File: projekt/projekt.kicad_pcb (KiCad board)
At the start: 2 copper layers, 28 parts, among them J1 Conn_01x05, J2 Conn_01x04, J4 87583-0010RHLF, J5 10118192-0001LF, U1 MAX17048G_T10, U2 TPS61022RWUT, U3 MCP73871-2CCI_ML

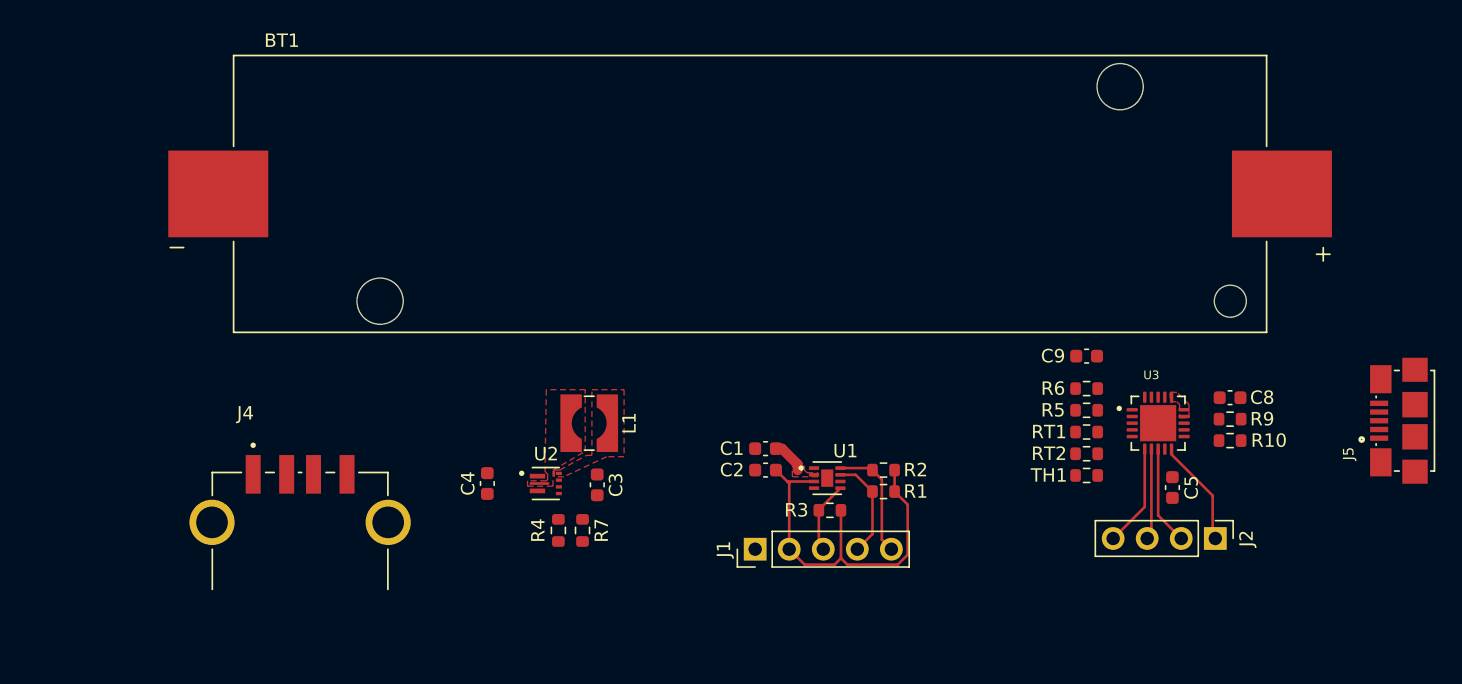
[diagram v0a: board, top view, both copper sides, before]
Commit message: MAIN: wersja pierwsza 19.04.
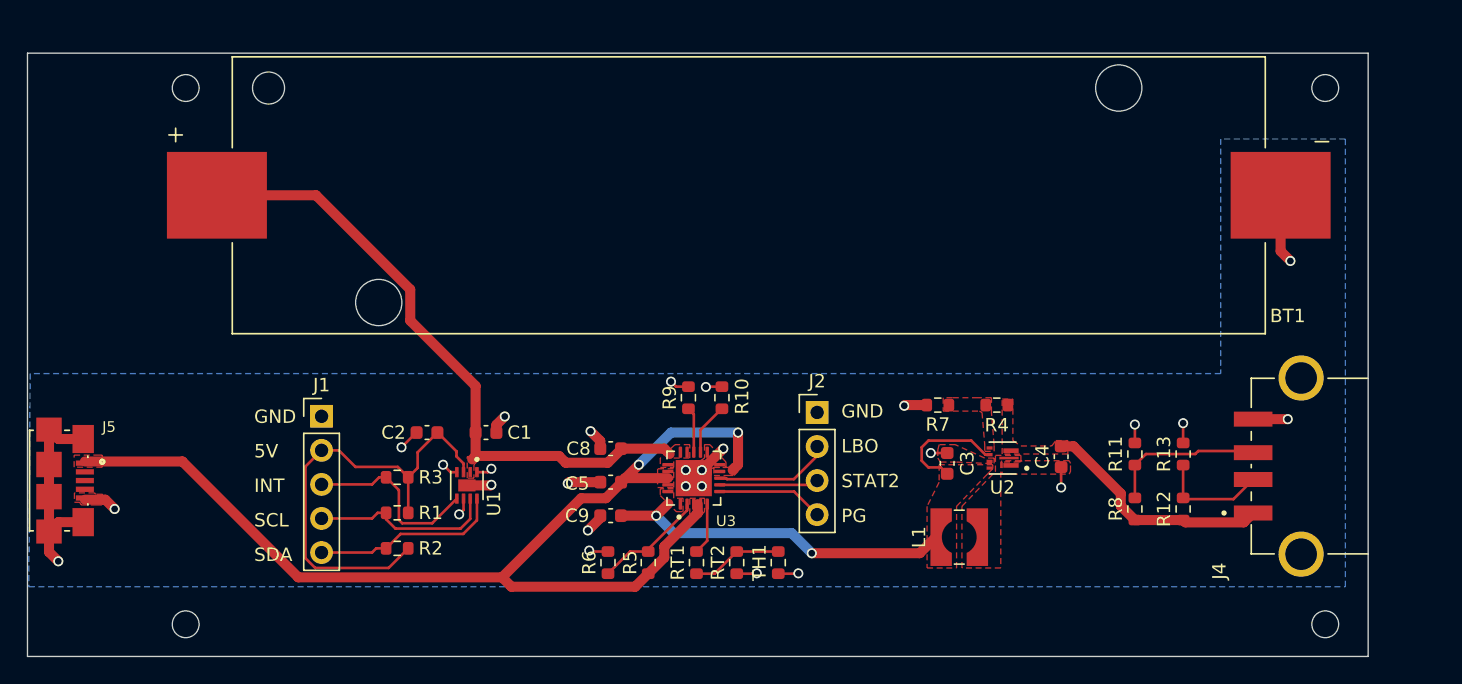
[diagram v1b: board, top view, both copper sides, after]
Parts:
- added R11: R, Resistor_SMD:R_0603_1608Metric, F.Cu at (166.2, 72.9)
- added R12: R, Resistor_SMD:R_0603_1608Metric, F.Cu at (169.8, 77.0)
- added R13: R, Resistor_SMD:R_0603_1608Metric, F.Cu at (169.8, 72.9)
- added R8: R, Resistor_SMD:R_0603_1608Metric, F.Cu at (166.2, 77.0)
- added REF**: MountingHole_2mm, MountingHole:MountingHole_2mm, F.Cu at (180.4, 45.6)
- added REF**: MountingHole_2mm, MountingHole:MountingHole_2mm, F.Cu at (95.4, 85.6)
- added REF**: MountingHole_2mm, MountingHole:MountingHole_2mm, F.Cu at (95.4, 45.6)
- added REF**: MountingHole_2mm, MountingHole:MountingHole_2mm, F.Cu at (180.4, 85.6)
- moved J5 96.6 mm to (87.9, 74.9), turned to -90 degrees
- moved J4 74.8 mm to (178.6, 73.8), turned to 90 degrees
- moved C8 46.4 mm to (127.1, 72.5), turned to 180 degrees
- moved C4 42.8 mm to (160.7, 73.1), turned to -90 degrees
- moved C5 41.9 mm to (127.1, 75.0), turned to 180 degrees
- moved R9 40.4 mm to (132.9, 68.7), turned to 90 degrees
- moved R10 38.0 mm to (135.4, 68.7), turned to 90 degrees
- moved R6 38.0 mm to (126.9, 81.0), turned to -90 degrees
- moved C9 37.4 mm to (127.1, 77.5)
- moved R2 36.7 mm to (111.2, 79.9)
- moved R1 36.3 mm to (111.2, 77.3)
- moved U3 34.9 mm to (133.3, 74.7), turned to 90 degrees
- moved R5 34.6 mm to (129.9, 81.0), turned to 90 degrees
- moved U2 34.1 mm to (156.3, 73.2), turned to 180 degrees
- moved R4 34.0 mm to (155.9, 69.2), turned to 180 degrees
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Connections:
- J4 pad 02: unconnected-(J4-D--Pad02) -> /D-
- J4 pad 03: unconnected-(J4-D+-Pad03) -> /D+
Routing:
- net +5V_CHARGE: track 0.00 -> 81.7 mm, vias 0 -> 2
- net GND: track 8.02 -> 57.8 mm, vias 0 -> 28
- net +BATT: track 2.54 -> 47.4 mm
- net V_LOAD: track 0.00 -> 35.4 mm, vias 0 -> 2
- net +5V_OUT: track 0.00 -> 17.5 mm
- net /D+: track 0.00 -> 11.8 mm
- net /INT: track 5.35 -> 13.8 mm
- net Net-(U3-VPCC): track 0.00 -> 8.42 mm
- net /D-: track 0.00 -> 8.41 mm
- net Net-(RT1-Pad2): track 0.00 -> 6.78 mm
- net V_IN_FG: track 28.6 -> 35.1 mm
- net /SCL: track 7.68 -> 13.8 mm
- net /SDA: track 8.94 -> 14.2 mm
- net Net-(U3-PROG3): track 0.00 -> 3.92 mm
- net Net-(U3-THERM): track 0.00 -> 3.87 mm
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- added copper zone on F.Cu, net +5V_CHARGE
- added copper zone on F.Cu, net +5V_OUT
- added copper zone on B.Cu, net GND
- added copper zone on F.Cu, net GND
- added copper zone on F.Cu, net Net-(U2-FB)
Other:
- board outline added: 100 x 45 mm
- board text added: "5V"
- board text added: "GND"
- board text added: "INT"
- board text added: "LBO"
- board text added: "PG"
- board text added: "SCL"
- board text added: "SDA"
- board text added: "STAT2"
